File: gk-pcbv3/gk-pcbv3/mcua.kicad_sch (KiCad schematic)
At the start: 20 parts, among them J12 Conn_01x03, SW1 SW_Push, U4 STM32H7S7L8H6H, Y2 32.768kHz R26-32.768-12.5

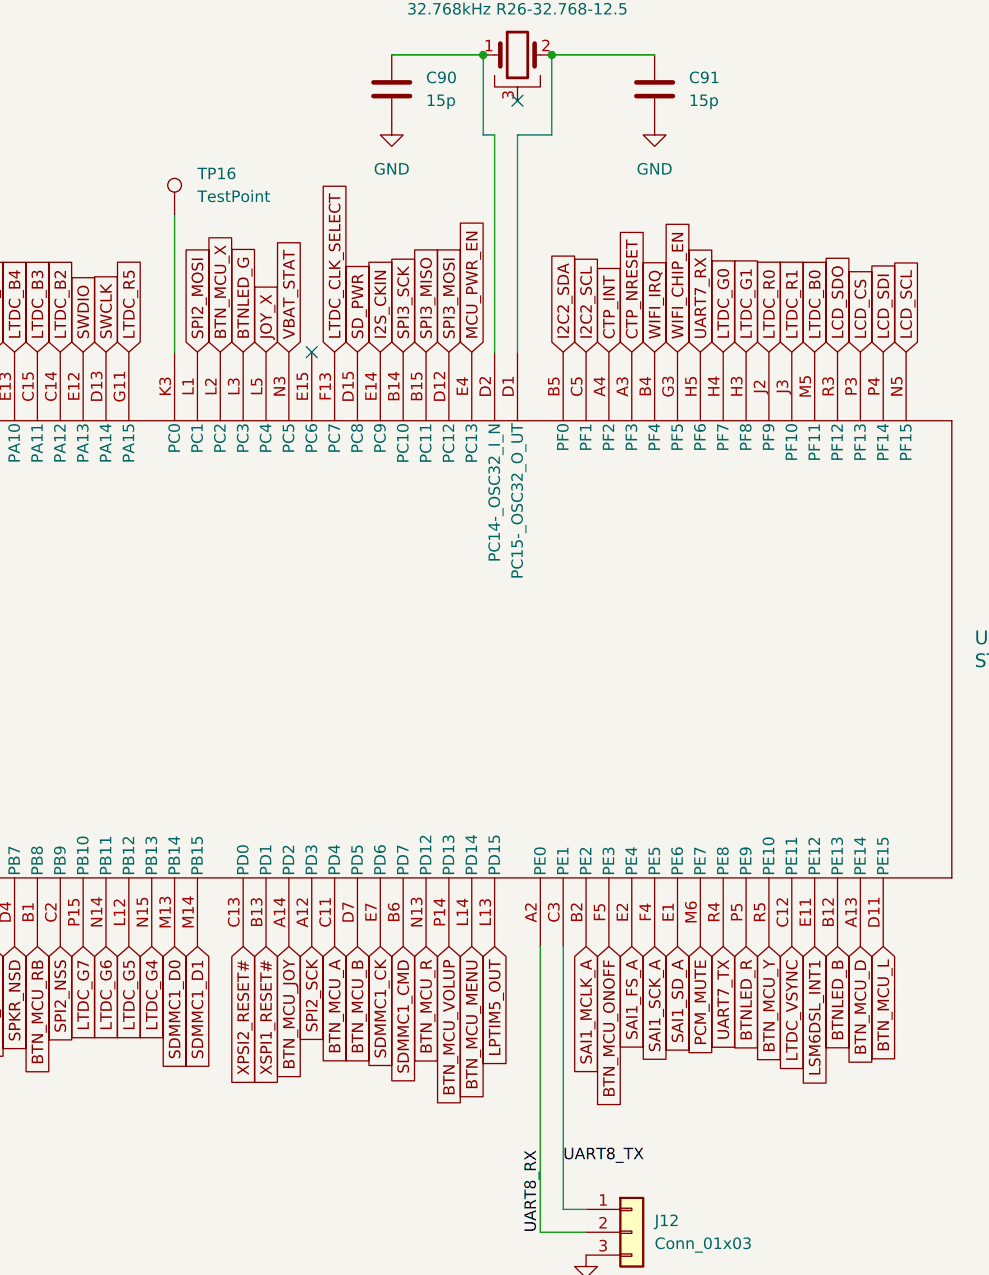
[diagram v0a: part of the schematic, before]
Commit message: new gerbers
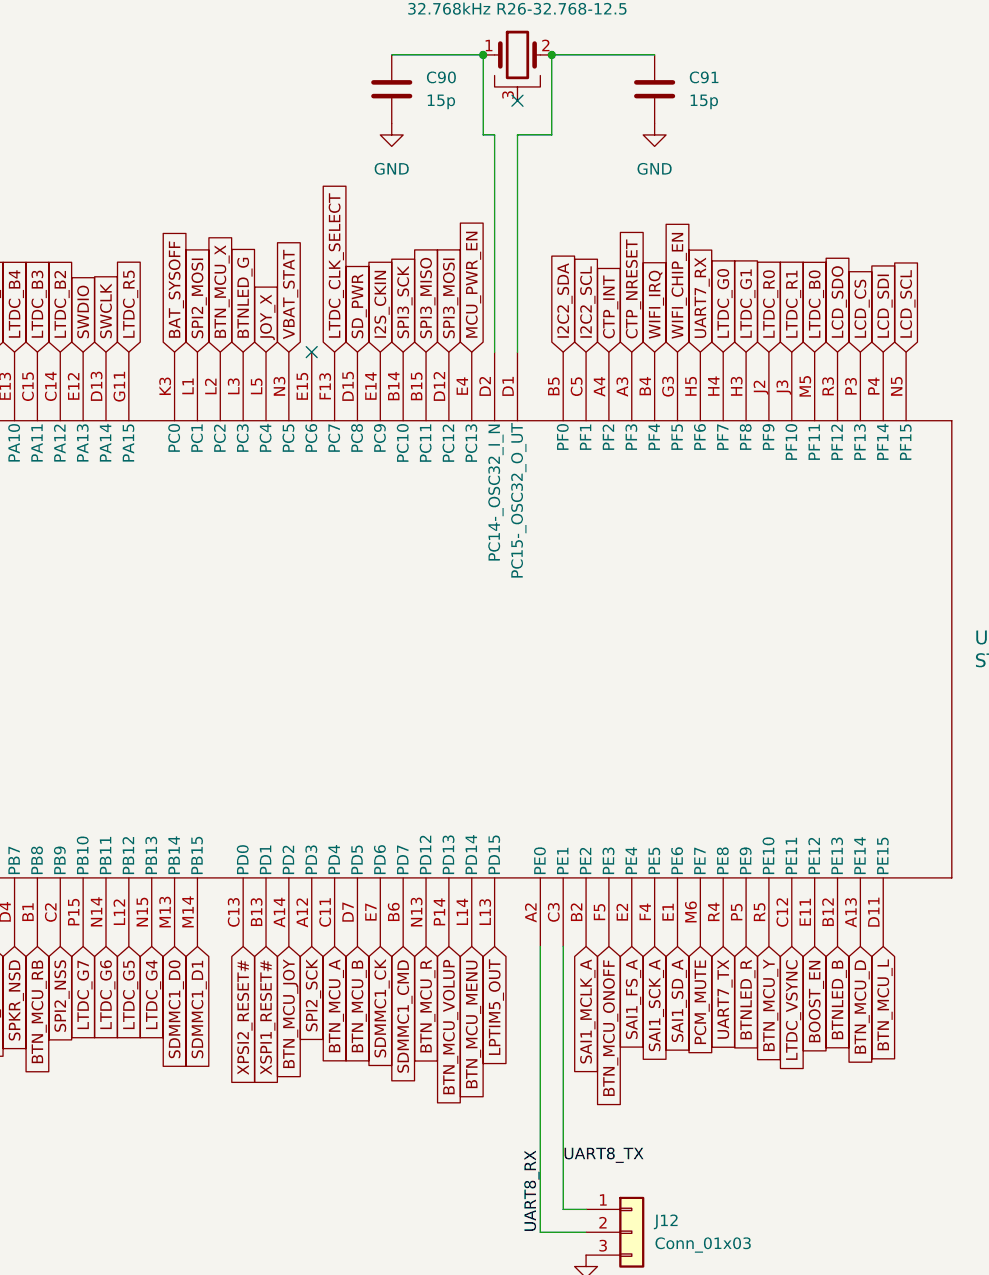
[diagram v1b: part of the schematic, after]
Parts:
- removed TP16: TestPoint, Connector_PinHeader_2.54mm:PinHeader_1x01_P2.54mm_Vertical, symbol Connector:TestPoint
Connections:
- net BAT_SYSOFF: now reaches U4.K3 (PC0)
- net LSM6DSL_INT1 renamed BOOST_EN
